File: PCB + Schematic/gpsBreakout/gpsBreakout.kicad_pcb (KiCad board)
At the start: 2 copper layers, 24.8 x 26.5 mm, 17 parts, among them J1 Header, U1 ATGM336H, U2 AT24CS32-STUM, U3 AT2659

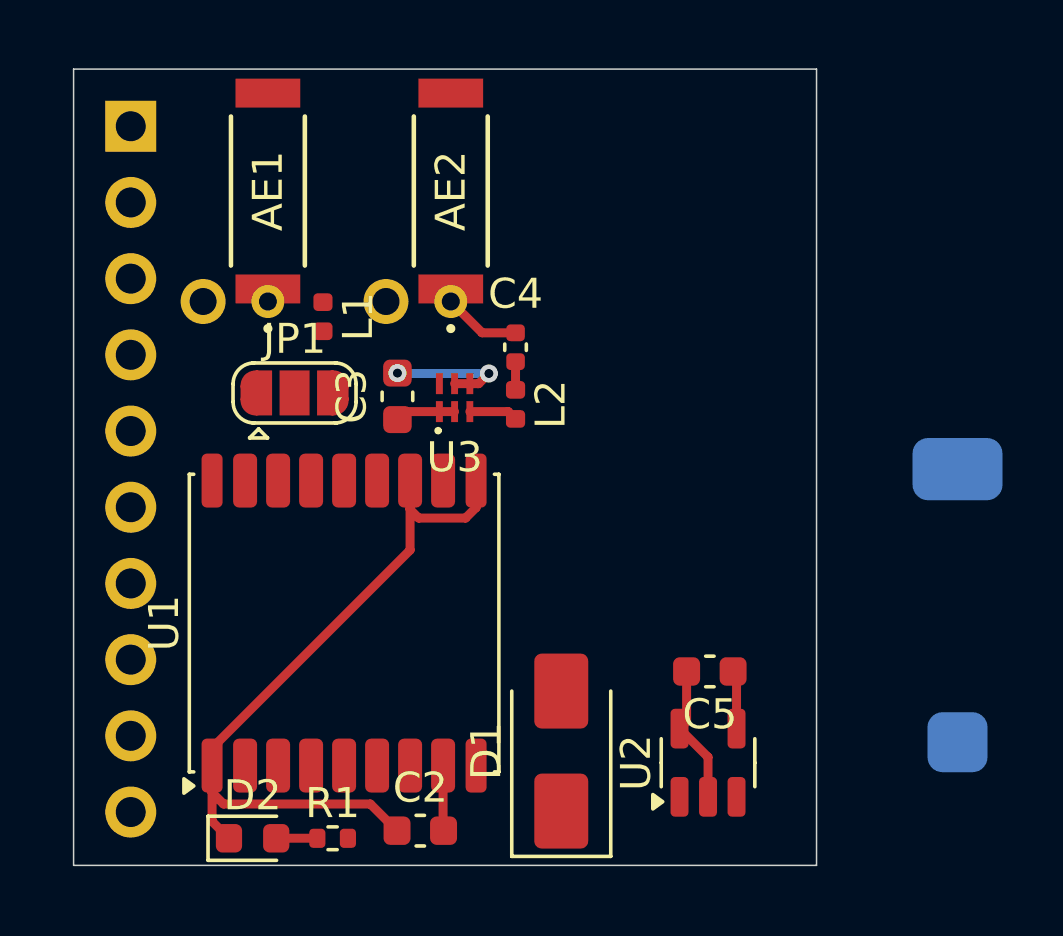
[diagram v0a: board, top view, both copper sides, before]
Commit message: Finished board
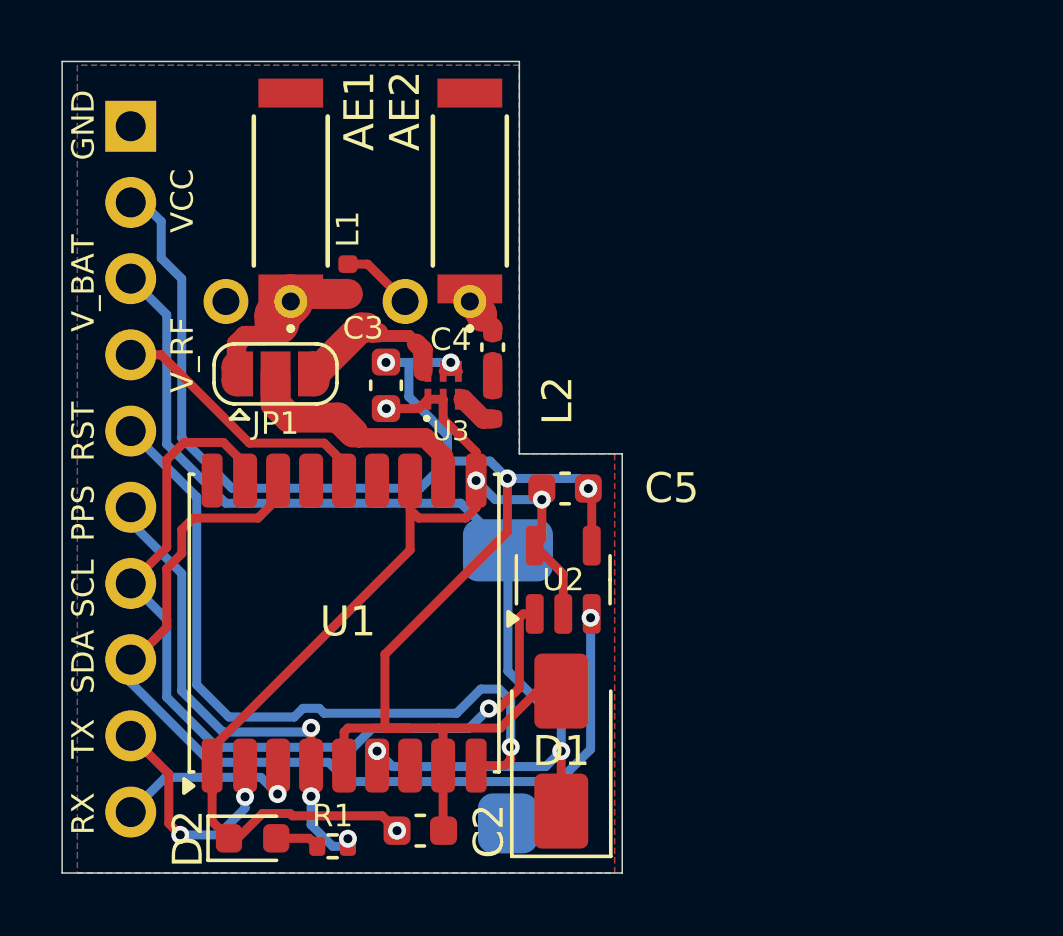
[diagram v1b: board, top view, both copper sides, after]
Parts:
- moved BT1 15.2 mm to (154.6, 102.8)
- moved U2 7.78 mm to (156.4, 94.6)
- moved C5 7.78 mm to (156.5, 91.6)
- moved L1 1.52 mm to (149.2, 84.6), turned to 90 degrees
- moved JP1 0.90 mm to (146.8, 87.8)
- moved AE1 0.76 mm to (147.3, 81.7)
- moved C4 0.76 mm to (154.1, 86.9)
- moved L2 0.76 mm to (154.1, 88.8)
- moved AE2 0.63 mm to (153.3, 81.7)
- moved U3 0.56 mm to (152.4, 88.1)
- moved C3 0.53 mm to (150.5, 88.1)
- moved R1 0.27 mm to (148.7, 103.5)
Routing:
- net +3.3V: track 8.47 -> 57.1 mm, vias 2 -> 4
- net VBAT: track 0.00 -> 35.3 mm, vias 0 -> 2
- net SDA: track 0.00 -> 31.8 mm, vias 0 -> 1
- net SCL: track 0.00 -> 28.8 mm, vias 0 -> 1
- net RESET: track 0.00 -> 24.2 mm, vias 0 -> 1
- net PPS: track 0.00 -> 16.5 mm, vias 0 -> 3
- net VCC_RF: track 0.00 -> 9.19 mm
- net RF: track 0.00 -> 8.85 mm
- net TX: track 0.00 -> 7.94 mm, vias 0 -> 2
- net PASSIVE: track 0.00 -> 6.13 mm
- net GND: track 33.5 -> 39.1 mm, vias 0 -> 4
- net RX: track 0.00 -> 5.61 mm, vias 0 -> 1
- net ACTIVE: track 0.00 -> 5.60 mm
- net Net-(AE2-FEED): track 2.59 -> 2.06 mm
- added copper zone on B.Cu, net GND
- added copper zone on F.Cu, net GND
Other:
- board size 24.8 x 26.5 mm -> 18.7 x 27.1 mm
- board text added: "Designed by Charles Nicholson, June 2024"
- board text added: "GND"
- board text added: "JLCJLCJLCJLC"
- board text added: "JP1: 1 = passive, 3 = active"
- board text added: "Made with support of Hack Club and NEWBS"
- board text added: "PPS"
- board text added: "RST"
- board text added: "RX"
- board text added: "SCL"
- board text added: "SDA"
- board text added: "TX"
- board text added: "VCC"
- board text added: "V_BAT"
- board text added: "V_RF"

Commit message: Folding glider, plus some PCB stuff from later
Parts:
- AE1, AE2: footprint 1575AT43A0040E:ANT_1575AT_JOT-L -> footprints:ANT_1575AT_JOT-L
- BT1: footprint Battery:MS621R -> footprints:MS621R
- C2, C3, C5: footprint Capacitor_SMD:C_0603_1608Metric -> footprints:C_0603_1608Metric
- C4: footprint Capacitor_SMD:C_0402_1005Metric -> footprints:C_0402_1005Metric
- D1: footprint Diode_SMD:D_SMA -> footprints:D_SMA
- D2: footprint LED_SMD:LED_0603_1608Metric -> footprints:LED_0603_1608Metric
- J1: footprint Connector_PinHeader_2.54mm:PinHeader_1x10_P2.54mm_Vertical -> footprints:PinHeader_1x10_P2.54mm_Vertical
- JP1: footprint Jumper:SolderJumper-3_P1.3mm_Open_RoundedPad1.0x1.5mm -> footprints:SolderJumper-3_P1.3mm_Open_RoundedPad1.0x1.5mm
- L1, L2: footprint Inductor_SMD:L_0402_1005Metric -> footprints:L_0402_1005Metric
- R1: footprint Resistor_SMD:R_0402_1005Metric -> footprints:R_0402_1005Metric
- U1: footprint RF_GPS:ATGM336H -> footprints:ATGM336H
- U2: footprint Package_TO_SOT_SMD:SOT-23-5 -> footprints:SOT-23-5
- U3: footprint AT2659:DFN150X100X80-6N -> footprints:DFN150X100X80-6N
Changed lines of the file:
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@@
 	(net 16 "ACTIVE")
 	(net 17 "Net-(U3-RF_IN)")
-	(footprint "1575AT43A0040E:ANT_1575AT_JOT-L"
+	(footprint "footprints:ANT_1575AT_JOT-L"
 		(layer "F.Cu")
 		(at 147.32 81.661 90)
@@
 			)
 		)
-		(property "Footprint" "1575AT43A0040E:ANT_1575AT_JOT-L"
+		(property "Footprint" "footprints:ANT_1575AT_JOT-L"
 			(at 0 0 90)
 			(unlocked yes)
@@
 		)
 	)
-	(footprint "LED_SMD:LED_0603_1608Metric"
+	(footprint "footprints:LED_0603_1608Metric"
 		(layer "F.Cu")
 		(at 146.048 103.237)
@@
 			)
 		)
-		(property "Footprint" "LED_SMD:LED_0603_1608Metric"
+		(property "Footprint" "footprints:LED_0603_1608Metric"
 			(at 0 0 0)
 			(unlocked yes)
@@
 			(pintype "passive")
 		)
-		(model "${KICAD8_3DMODEL_DIR}/LED_SMD.3dshapes/LED_0603_1608Metric.wrl"
+		(model "${KIPRJMOD}/packages3D/LED_0603_1608Metric.wrl"
 			(offset
 				(xyz 0 0 0)
@@
 		)
 	)
-	(footprint "Capacitor_SMD:C_0603_1608Metric"
+	(footprint "footprints:C_0603_1608Metric"
 		(layer "F.Cu")
 		(at 150.495 88.138 -90)
@@
 			)
 		)
-		(property "Footprint" "Capacitor_SMD:C_0603_1608Metric"
+		(property "Footprint" "footprints:C_0603_1608Metric"
 			(at 0 0 -90)
 			(unlocked yes)
@@
 			(pintype "passive")
 		)
-		(model "${KICAD8_3DMODEL_DIR}/Capacitor_SMD.3dshapes/C_0603_1608Metric.wrl"
+		(model "${KIPRJMOD}/packages3D/C_0603_1608Metric.wrl"
 			(offset
 				(xyz 0 0 0)
@@
 		)
 	)
-	(footprint "1575AT43A0040E:ANT_1575AT_JOT-L"
+	(footprint "footprints:ANT_1575AT_JOT-L"
 		(layer "F.Cu")
 		(at 153.289 81.661 90)
@@
 			)
 		)
-		(property "Footprint" "1575AT43A0040E:ANT_1575AT_JOT-L"
+		(property "Footprint" "footprints:ANT_1575AT_JOT-L"
 			(at 0 0 90)
 			(unlocked yes)
@@
 		)
 	)
-	(footprint "Inductor_SMD:L_0402_1005Metric"
+	(footprint "footprints:L_0402_1005Metric"
 		(layer "F.Cu")
 		(at 149.225 84.582 90)
@@
 		(tags "inductor")
 		(property "Reference" "L1"
-			(at 1.651 0 270)
+			(at 1.651 0 -90)
 			(layer "F.SilkS")
 			(effects
@@
 			)
 		)
-		(property "Footprint" "Inductor_SMD:L_0402_1005Metric"
+		(property "Footprint" "footprints:L_0402_1005Metric"
 			(at 0 0 90)
 			(unlocked yes)
@@
 			(pintype "passive")
 		)
-		(model "${KICAD8_3DMODEL_DIR}/Inductor_SMD.3dshapes/L_0402_1005Metric.wrl"
+		(model "${KIPRJMOD}/packages3D/L_0402_1005Metric.wrl"
 			(offset
 				(xyz 0 0 0)
@@
 		)
 	)
-	(footprint "Jumper:SolderJumper-3_P1.3mm_Open_RoundedPad1.0x1.5mm"
+	(footprint "footprints:SolderJumper-3_P1.3mm_Open_RoundedPad1.0x1.5mm"
 		(layer "F.Cu")
 		(at 146.812 87.757)
@@
 			)
 		)
-		(property "Footprint" "Jumper:SolderJumper-3_P1.3mm_Open_RoundedPad1.0x1.5mm"
+		(property "Footprint" "footprints:SolderJumper-3_P1.3mm_Open_RoundedPad1.0x1.5mm"
 			(at 0 0 0)
 			(unlocked yes)
@@
 		)
 	)
-	(footprint "RF_GPS:ATGM336H"
+	(footprint "footprints:ATGM336H"
 		(layer "F.Cu")
 		(at 149.098 96.063 90)
@@
 			)
 		)
-		(property "Footprint" "RF_GPS:ATGM336H"
+		(property "Footprint" "footprints:ATGM336H"
 			(at 0 0 90)
 			(unlocked yes)
@@
 			(roundrect_rratio 0.25)
 		)
-		(model "${KICAD8_3DMODEL_DIR}/RF_GPS.3dshapes/ublox_MAX.wrl"
+		(model "${KIPRJMOD}/packages3D/ublox_MAX.wrl"
 			(offset
 				(xyz 0 0 0)
@@
 		)
 	)
-	(footprint "Capacitor_SMD:C_0603_1608Metric"
+	(footprint "footprints:C_0603_1608Metric"
 		(layer "F.Cu")
 		(at 156.464 91.578 180)
@@
 			)
 		)
-		(property "Footprint" "Capacitor_SMD:C_0603_1608Metric"
+		(property "Footprint" "footprints:C_0603_1608Metric"
 			(at 0 0 180)
 			(unlocked yes)
@@
 			(pintype "passive")
 		)
-		(model "${KICAD8_3DMODEL_DIR}/Capacitor_SMD.3dshapes/C_0603_1608Metric.wrl"
+		(model "${KIPRJMOD}/packages3D/C_0603_1608Metric.wrl"
 			(offset
 				(xyz 0 0 0)
@@
 		)
 	)
-	(footprint "Capacitor_SMD:C_0402_1005Metric"
+	(footprint "footprints:C_0402_1005Metric"
 		(layer "F.Cu")
 		(at 154.051 86.868 -90)
@@
 			)
 		)
-		(property "Footprint" "Capacitor_SMD:C_0402_1005Metric"
+		(property "Footprint" "footprints:C_0402_1005Metric"
 			(at 0 0 -90)
 			(unlocked yes)
@@
 			(pintype "passive")
 		)
-		(model "${KICAD8_3DMODEL_DIR}/Capacitor_SMD.3dshapes/C_0402_1005Metric.wrl"
+		(model "${KIPRJMOD}/packages3D/C_0402_1005Metric.wrl"
 			(offset
 				(xyz 0 0 0)
@@
 		)
 	)
-	(footprint "Inductor_SMD:L_0402_1005Metric"
+	(footprint "footprints:L_0402_1005Metric"
 		(layer "F.Cu")
 		(at 154.051 88.773 -90)
@@
 			)
 		)
-		(property "Footprint" "Inductor_SMD:L_0402_1005Metric"
+		(property "Footprint" "footprints:L_0402_1005Metric"
 			(at 0 0 -90)
 			(unlocked yes)
@@
 			(pintype "passive")
 		)
-		(model "${KICAD8_3DMODEL_DIR}/Inductor_SMD.3dshapes/L_0402_1005Metric.wrl"
+		(model "${KIPRJMOD}/packages3D/L_0402_1005Metric.wrl"
 			(offset
 				(xyz 0 0 0)
@@
 		)
 	)
-	(footprint "Diode_SMD:D_SMA"
+	(footprint "footprints:D_SMA"
 		(layer "F.Cu")
 		(at 156.337 100.33 90)
@@
 			)
 		)
-		(property "Footprint" "Diode_SMD:D_SMA"
+		(property "Footprint" "footprints:D_SMA"
 			(at 0 0 90)
 			(unlocked yes)
@@
 			(pintype "passive")
 		)
-		(model "${KICAD8_3DMODEL_DIR}/Diode_SMD.3dshapes/D_SMA.wrl"
+		(model "${KIPRJMOD}/packages3D/D_SMA.wrl"
 			(offset
 				(xyz 0 0 0)
@@
 		)
 	)
-	(footprint "Capacitor_SMD:C_0603_1608Metric"
+	(footprint "footprints:C_0603_1608Metric"
 		(layer "F.Cu")
 		(at 151.638 102.983)
@@
 			)
 		)
-		(property "Footprint" "Capacitor_SMD:C_0603_1608Metric"
+		(property "Footprint" "footprints:C_0603_1608Metric"
 			(at 0 0 0)
 			(unlocked yes)
@@
 			(pintype "passive")
 		)
-		(model "${KICAD8_3DMODEL_DIR}/Capacitor_SMD.3dshapes/C_0603_1608Metric.wrl"
+		(model "${KIPRJMOD}/packages3D/C_0603_1608Metric.wrl"
 			(offset
 				(xyz 0 0 0)
@@
 		)
 	)
-	(footprint "Package_TO_SOT_SMD:SOT-23-5"
+	(footprint "footprints:SOT-23-5"
 		(layer "F.Cu")
 		(at 156.403 94.6205 90)
@@
 			)
 		)
-		(property "Footprint" "Package_TO_SOT_SMD:SOT-23-5"
+		(property "Footprint" "footprints:SOT-23-5"
 			(at 0 0 90)
 			(unlocked yes)
@@
 			(pintype "input")
 		)
-		(model "${KICAD8_3DMODEL_DIR}/Package_TO_SOT_SMD.3dshapes/SOT-23-5.wrl"
+		(model "${KIPRJMOD}/packages3D/SOT-23-5.wrl"
 			(offset
 				(xyz 0 0 0)
@@
 		)
 	)
-	(footprint "AT2659:DFN150X100X80-6N"
+	(footprint "footprints:DFN150X100X80-6N"
 		(layer "F.Cu")
 		(at 152.4 88.138 90)
@@
 			)
 		)
-		(property "Footprint" "AT2659:DFN150X100X80-6N"
+		(property "Footprint" "footprints:DFN150X100X80-6N"
 			(at 0 0 90)
 			(unlocked yes)
@@
 		)
 	)
-	(footprint "Resistor_SMD:R_0402_1005Metric"
+	(footprint "footprints:R_0402_1005Metric"
 		(layer "F.Cu")
 		(at 148.715 103.505)
@@
 			)
 		)
-		(property "Footprint" "Resistor_SMD:R_0402_1005Metric"
+		(property "Footprint" "footprints:R_0402_1005Metric"
 			(at 0 0 0)
 			(unlocked yes)
@@
 			(pintype "passive")
 		)
-		(model "${KICAD8_3DMODEL_DIR}/Resistor_SMD.3dshapes/R_0402_1005Metric.wrl"
+		(model "${KIPRJMOD}/packages3D/R_0402_1005Metric.wrl"
 			(offset
 				(xyz 0 0 0)
@@
 		)
 	)
-	(footprint "Connector_PinHeader_2.54mm:PinHeader_1x10_P2.54mm_Vertical"
+	(footprint "footprints:PinHeader_1x10_P2.54mm_Vertical"
 		(layer "B.Cu")
 		(at 141.986 79.502 180)
@@
 			)
 		)
-		(property "Footprint" "Connector_PinHeader_2.54mm:PinHeader_1x10_P2.54mm_Vertical"
+		(property "Footprint" "footprints:PinHeader_1x10_P2.54mm_Vertical"
 			(at 0 0 0)
 			(unlocked yes)
@@
 			(pintype "passive")
 		)
-		(model "${KICAD8_3DMODEL_DIR}/Connector_PinHeader_2.54mm.3dshapes/PinHeader_1x10_P2.54mm_Vertical.wrl"
+		(model "${KIPRJMOD}/packages3D/PinHeader_1x10_P2.54mm_Vertical.wrl"
 			(offset
 				(xyz 0 0 0)
@@
 		)
 	)
-	(footprint "Battery:MS621R"
+	(footprint "footprints:MS621R"
 		(layer "B.Cu")
 		(at 154.559 102.7615 90)
@@
 			)
 		)
-		(property "Footprint" "Battery:MS621R"
+		(property "Footprint" "footprints:MS621R"
 			(at 0 0 -90)
 			(unlocked yes)
